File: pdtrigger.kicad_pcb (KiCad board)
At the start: 4 copper layers, 56 x 53 mm, 91 parts, among them J1 Conn_01x04_Pin, J2 USB_C_Receptacle_USB2.0_16P, J3 Conn_01x02_Pin, Q1 DMP3098LSD-13, Q3 NMOS, SW1 SW_SPDT, SW2 SW_Push, U1 STM32F401RBT6, U2 CYPD3177-24LQXQ, U3 TERM_BLK, U4 SY8303AIC, Y1 16MHz

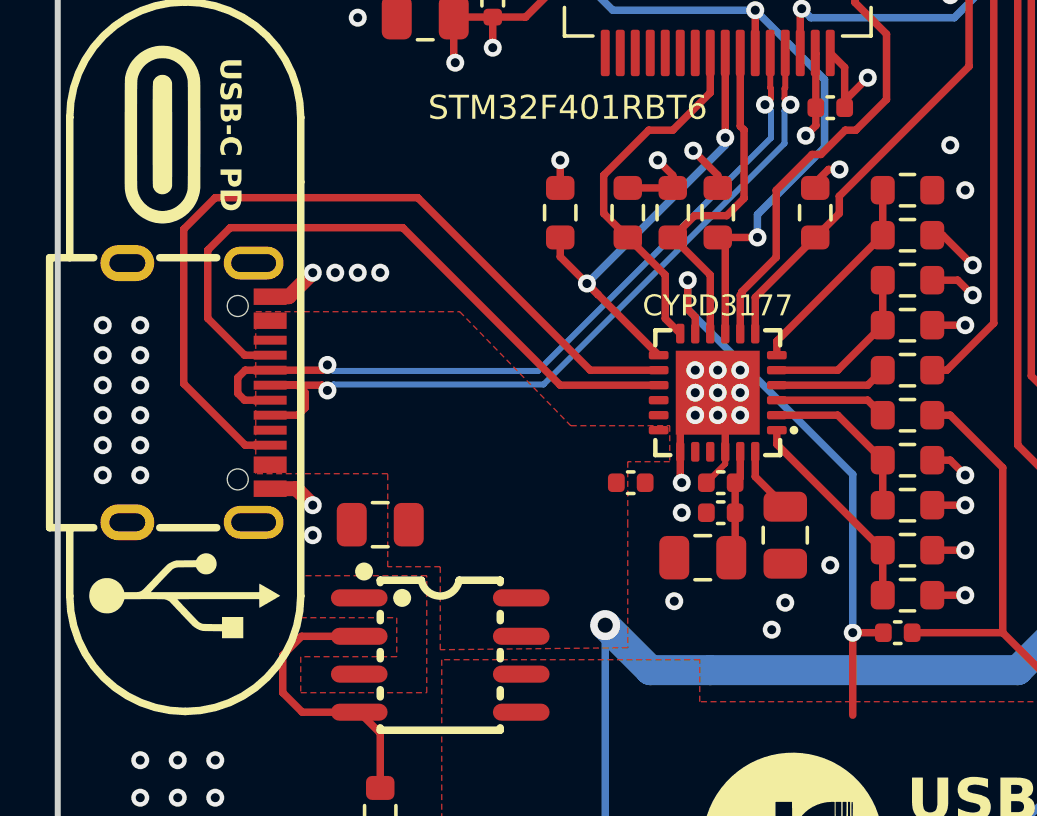
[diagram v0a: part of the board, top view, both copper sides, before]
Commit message: Changed as per design review
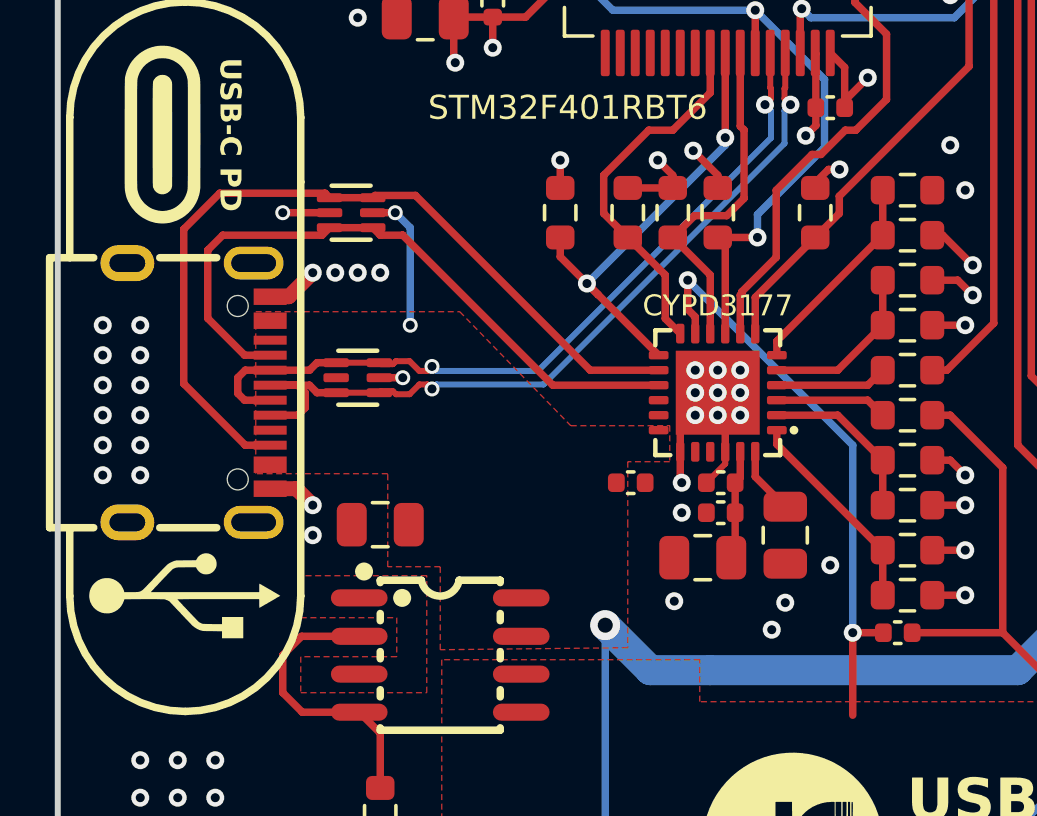
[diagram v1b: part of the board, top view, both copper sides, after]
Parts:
- added D8: USBLC6-2P6, libs:SOT-666-6_L1.6-W1.2-P0.50-LS1.6-BR, F.Cu at (136.5, 121.5)
- added D9: USBLC6-2P6, libs:SOT-666-6_L1.6-W1.2-P0.50-LS1.6-BR, F.Cu at (136.3, 116.0)
- renumbered TP2 to TP3, TP1 to TP3
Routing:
- net /VBUS: track 68.1 -> 72.9 mm, vias 4 -> 6
- net GND: track 36.2 -> 38.6 mm, vias 133 -> 135
